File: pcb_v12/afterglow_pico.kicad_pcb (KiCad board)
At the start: 2 copper layers, 57.5 x 57.5 mm, 40 parts, among them J1 Conn_02x17_Odd_Even, J2 Conn_02x17_Odd_Even, U1 74LS21, U2 7408, U3 SN74LVC245AN, U4 SN74LVC245AN, U5 SC0915, U6 74LS245, U7 74LS245, U8 74LS257, U9 74LS257

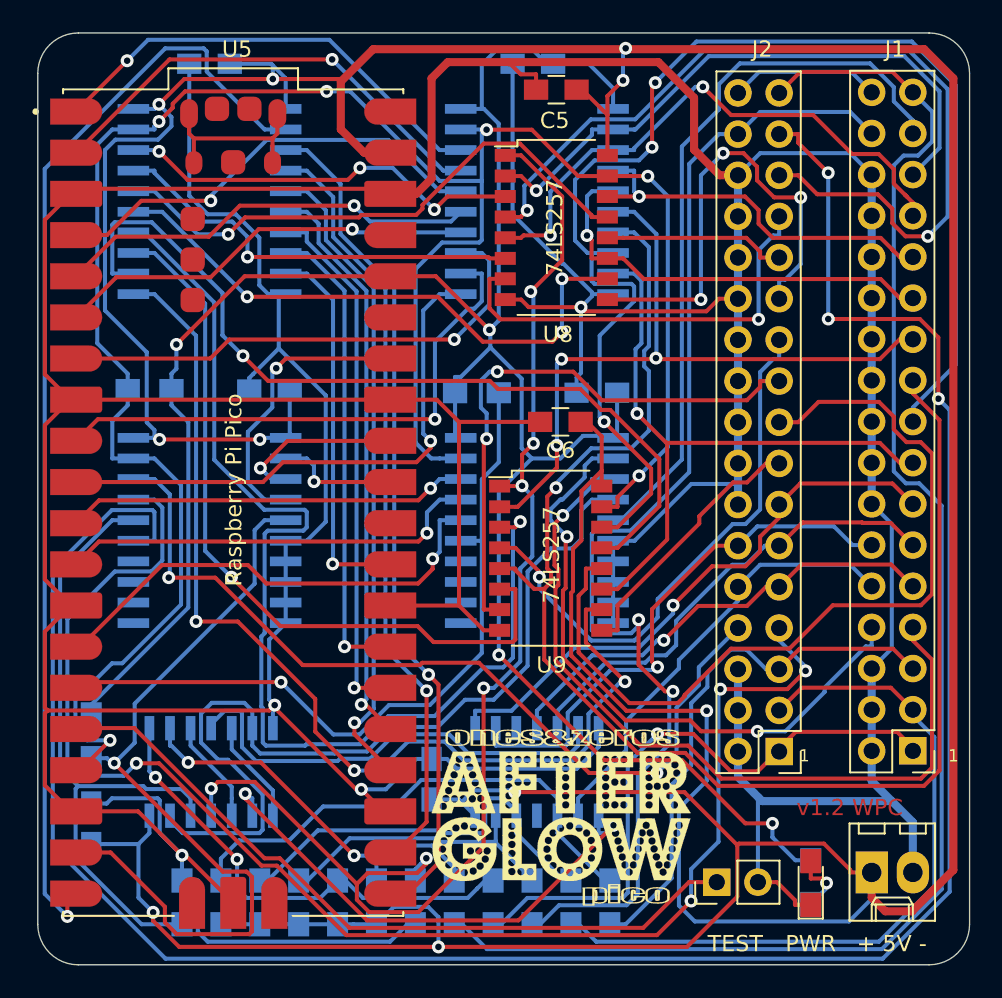
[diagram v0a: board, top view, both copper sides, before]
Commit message: JLCPCB production files
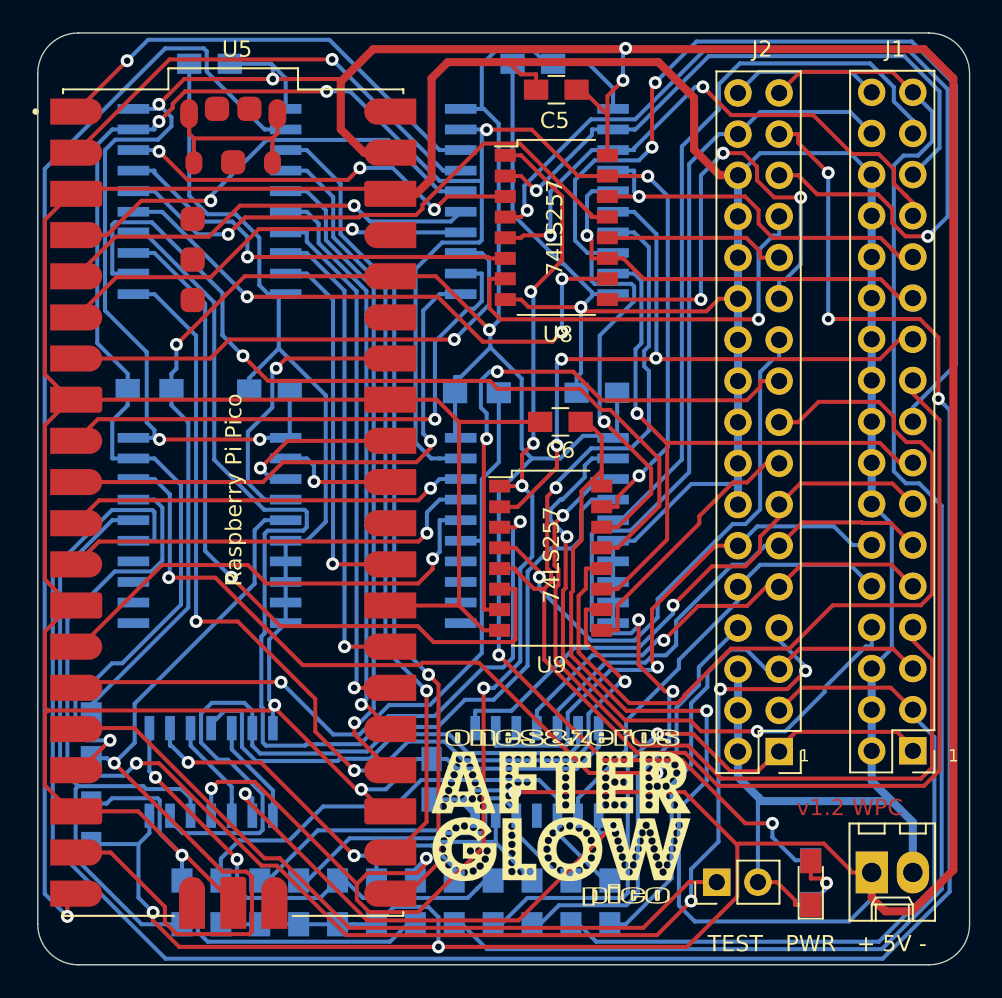
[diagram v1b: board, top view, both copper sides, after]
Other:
- net class Default removed
